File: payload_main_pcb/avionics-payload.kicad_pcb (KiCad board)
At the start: 2 copper layers, 69.8 x 80 mm, 41 parts, among them J1 USB_C_Receptacle_USB2.0, J2 Micro_SD_Card, J3 Conn_Coaxial, J4 Screw_Terminal_01x02, SW1 SW_Push, SW2 SW_Push, SW3 SW_Push, U1 ADIS16470AMLZ, U2 Teensy4.0, U3 74LS14, U4 RFM96W-433S2, U5 LT1129-3.3_SOT223, U6 MS5607-02BA, U7 ublox_SAM-M8Q

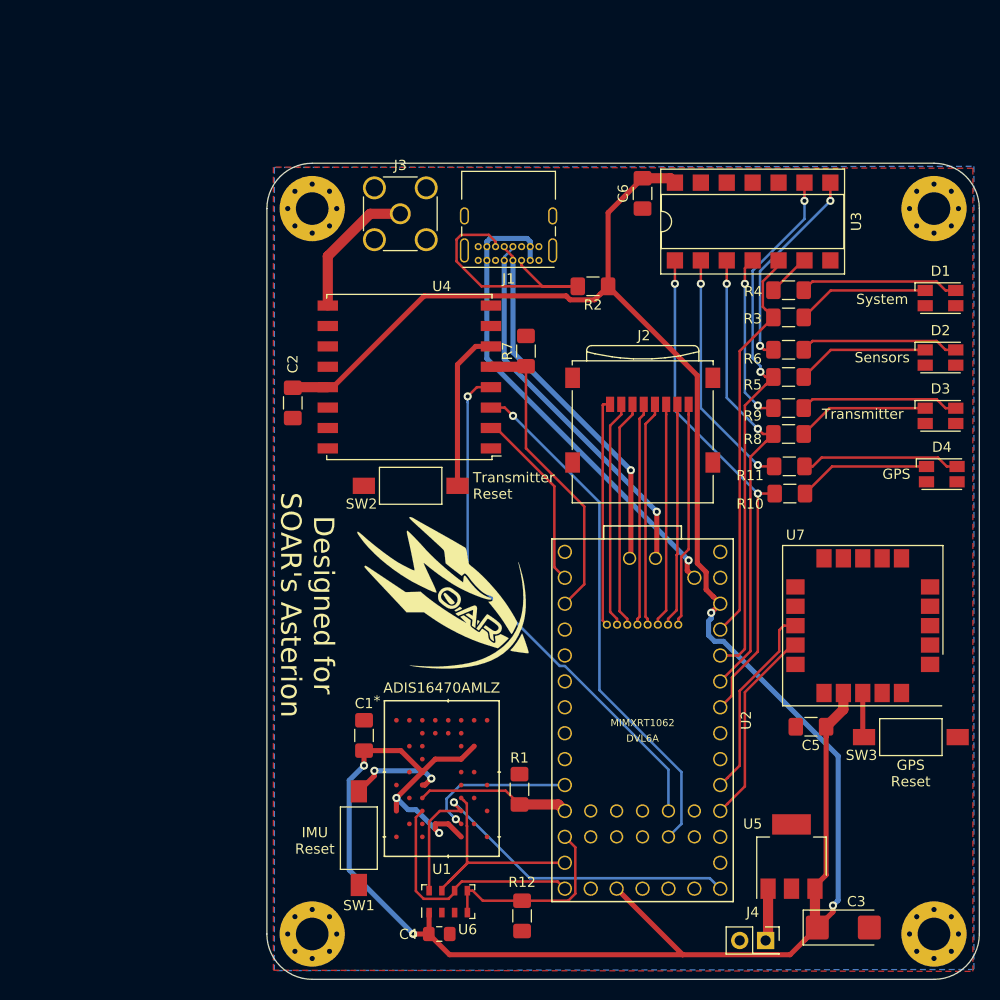
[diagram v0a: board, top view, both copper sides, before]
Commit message: PCB REV A
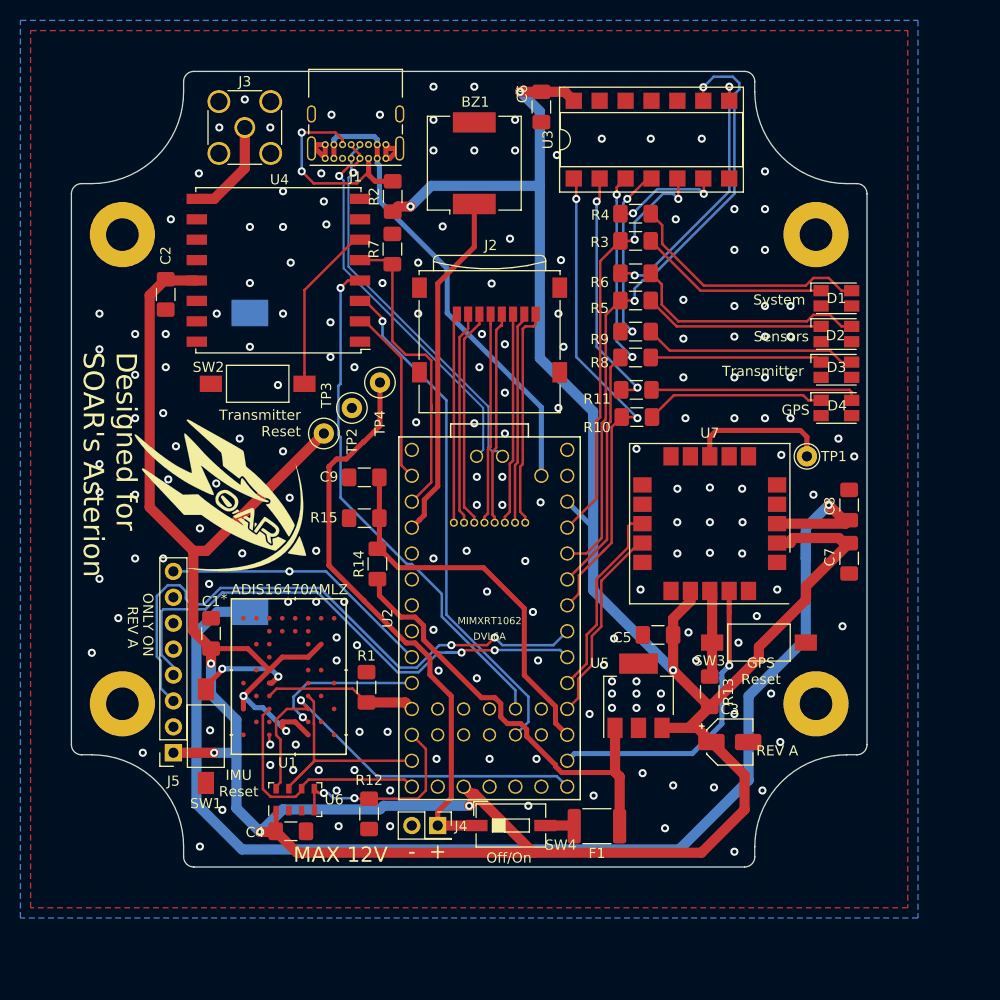
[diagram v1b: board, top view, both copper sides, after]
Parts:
- removed the REF** at (54.6, 44.5)
- removed the REF** at (54.6, 115.6)
- removed the REF** at (115.6, 44.5)
- removed the REF** at (115.6, 115.6)
- added BT1: Battery_Cell, Battery:BatteryHolder_Keystone_1060_1x2032, B.Cu at (48.5, 69.3)
- added BZ1: Buzzer, Buzzer_Beeper:Buzzer_CUI_CPT-9019S-SMT, F.Cu at (70.5, 40.0)
- added C7: 100nF, Capacitor_SMD:C_1206_3216Metric_Pad1.42x1.75mm_HandSolder, F.Cu at (107.2, 78.7)
- added C8: 100nF, Capacitor_SMD:C_1206_3216Metric_Pad1.42x1.75mm_HandSolder, F.Cu at (107.2, 73.5)
- added C9: 100nF, Capacitor_SMD:C_1206_3216Metric_Pad1.42x1.75mm_HandSolder, F.Cu at (59.7, 70.8)
- added F1: Polyfuse, Fuse:Fuse_1812_4532Metric_Pad1.30x3.40mm_HandSolder, F.Cu at (82.5, 105.0)
- added J5: Conn_01x08, Connector_PinSocket_2.54mm:PinSocket_1x08_P2.54mm_Vertical, F.Cu at (41.0, 97.8)
- added R13: 11k, Resistor_SMD:R_1206_3216Metric_Pad1.42x1.75mm_HandSolder, F.Cu at (93.6, 91.8)
- added R14: 10M, Resistor_SMD:R_1206_3216Metric_Pad1.42x1.75mm_HandSolder, F.Cu at (61.0, 79.3)
- added R15: 3.3M, Resistor_SMD:R_1206_3216Metric_Pad1.42x1.75mm_HandSolder, F.Cu at (59.7, 74.8)
- added REF**: MountingHole_3.2mm_M3_Pad, MountingHole:MountingHole_3.2mm_M3_Pad, F.Cu at (104.0, 47.0)
- added REF**: MountingHole_3.2mm_M3_Pad, MountingHole:MountingHole_3.2mm_M3_Pad, F.Cu at (104.0, 93.0)
- added REF**: MountingHole_3.2mm_M3_Pad, MountingHole:MountingHole_3.2mm_M3_Pad, F.Cu at (36.0, 93.0)
- added REF**: MountingHole_3.2mm_M3_Pad, MountingHole:MountingHole_3.2mm_M3_Pad, F.Cu at (36.0, 47.0)
- added SW4: SW_SPST, Button_Switch_SMD:SW_DIP_SPSTx01_Slide_6.7x4.1mm_W6.73mm_P2.54mm_LowProfile_JPin, F.Cu at (74.1, 104.9)
- added TP1: TestPoint, Connector_Pin:Pin_D1.0mm_L10.0mm, F.Cu at (103.1, 68.7)
- added TP2: TestPoint, TestPoint:TestPoint_Loop_D2.50mm_Drill1.0mm, F.Cu at (58.5, 64.0)
- added TP3: TestPoint, TestPoint:TestPoint_Loop_D2.50mm_Drill1.0mm, F.Cu at (55.8, 66.5)
- added TP4: TestPoint, TestPoint:TestPoint_Loop_D2.50mm_Drill1.0mm, F.Cu at (61.2, 61.5)
- C3: footprint Capacitor_Tantalum_SMD:CP_EIA-6032-15_Kemet-U_Pad2.25x2.35mm_HandSolder -> Capacitor_SMD:CP_Elec_4x5.4
- C4: footprint Capacitor_SMD:C_0805_2012Metric_Pad1.15x1.40mm_HandSolder -> Capacitor_SMD:C_1206_3216Metric_Pad1.42x1.75mm_HandSolder
- moved J4 34.1 mm to (66.9, 104.9)
- moved Ref** 23.8 mm to (14.5, 104.8)
- moved U5 21.8 mm to (86.6, 92.2)
- moved R2 21.5 mm to (62.5, 43.3), turned to 90 degrees
- moved C3 21.3 mm to (95.5, 96.8)
- moved R1 18.0 mm to (59.9, 91.4)
- moved C1 18.0 mm to (44.7, 86.1)
- moved R12 18.0 mm to (60.2, 103.8)
- moved SW1 18.0 mm to (44.2, 96.2)
- moved SW2 18.0 mm to (49.3, 61.6)
- moved U1 18.0 mm to (52.3, 90.3)
- moved U2 18.0 mm to (72.0, 84.6)
- moved U7 18.0 mm to (93.6, 75.3)
- moved J1 18.0 mm to (61.8, 39.5)
- moved U6 18.0 mm to (52.9, 102.4)
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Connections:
- U2 pad 21: Net-(U2-Pad21) -> GPS_EXTINT
- U2 pad 22: Net-(U2-Pad22) -> BATT_SENSE
- U2 pad 25: Net-(U2-Pad25) -> SDA
- U2 pad 26: Net-(U2-Pad26) -> SCL
- U2 pad 4: Net-(U2-Pad4) -> BUZZER
- U2 pad 9: Net-(U2-Pad9) -> INT
- U5 pad 1: +BATT -> Net-(F1-Pad1)
- U7 pad 19: Net-(U7-Pad19) -> GPS_EXTINT
- U7 pad 2: Net-(U7-Pad2) -> +3V3
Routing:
- net Net-(BT1-Pad1): track 0.00 -> 123.5 mm, vias 0 -> 1
- net +3V3: track 251.5 -> 345.0 mm, vias 6 -> 9
- net SCL: track 0.00 -> 58.8 mm, vias 0 -> 2
- net SDA: track 0.00 -> 52.7 mm, vias 0 -> 2
- net +BATT: track 5.18 -> 55.9 mm
- net Net-(F1-Pad1): track 0.00 -> 43.8 mm
- net BATT_SENSE: track 0.00 -> 37.8 mm
- net BUZZER: track 0.00 -> 34.3 mm
- net GPS_EXTINT: track 0.00 -> 30.0 mm, vias 0 -> 1
- net INT: track 0.00 -> 26.9 mm, vias 0 -> 1
- net Net-(TP1-Pad1): track 0.00 -> 13.9 mm
- net GND: track 0.00 -> 10.2 mm, vias 0 -> 180
- net Net-(D1-Pad2): track 15.6 -> 24.5 mm
- net SensorStatus: track 52.9 -> 60.9 mm
- net Net-(D2-Pad2): track 15.6 -> 23.6 mm
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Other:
- board size 69.8 x 80 mm -> 78 x 78 mm
- board text added: "+"
- board text added: "-"
- board text added: "MAX 12V"
- board text added: "ONLY ON"
- board text added: "Off/On"
- board text added: "REV A"
